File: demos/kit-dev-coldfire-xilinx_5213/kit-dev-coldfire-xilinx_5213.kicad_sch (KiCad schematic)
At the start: 66 parts, among them Q101 3906, U101 74AHC1G14, U102 MCF5213-LQFP100, Y101 8MHz

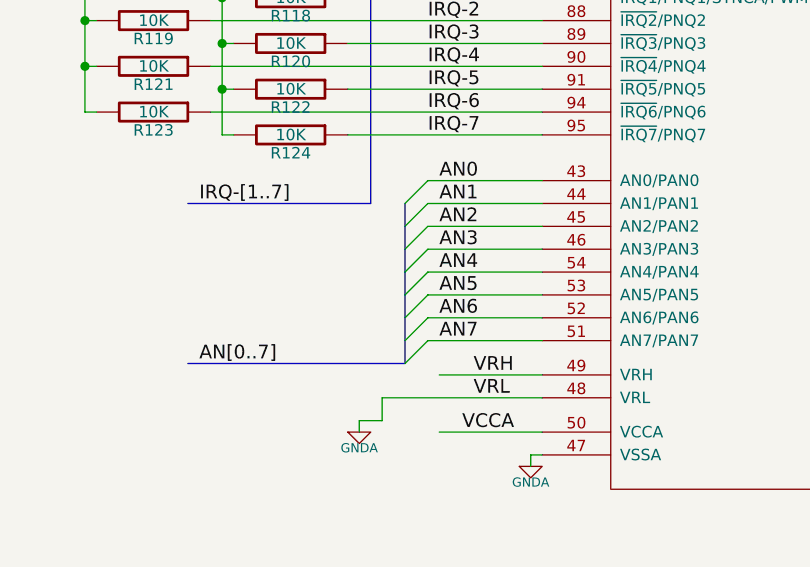
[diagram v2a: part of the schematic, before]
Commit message: Update demos
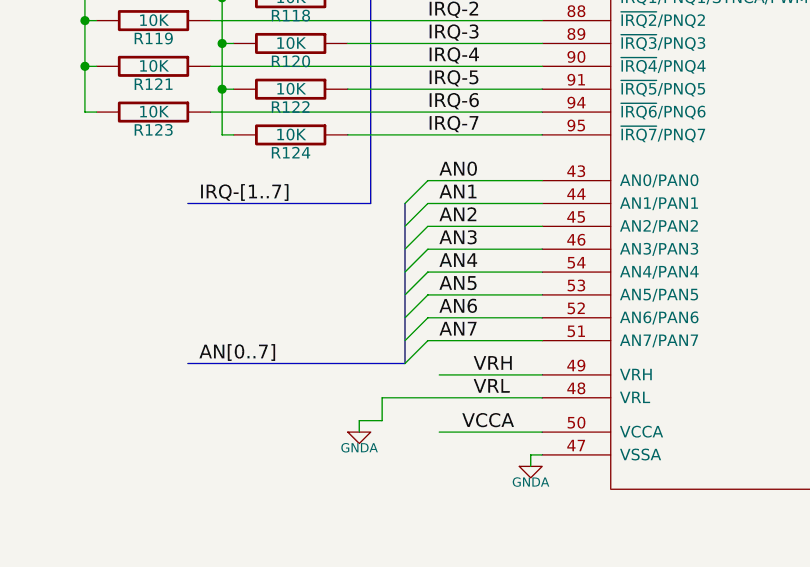
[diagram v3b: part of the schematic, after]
